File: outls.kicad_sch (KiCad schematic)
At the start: 6 parts, among them U5001 VNLD5160TR-E, U5002 VNLD5160TR-E

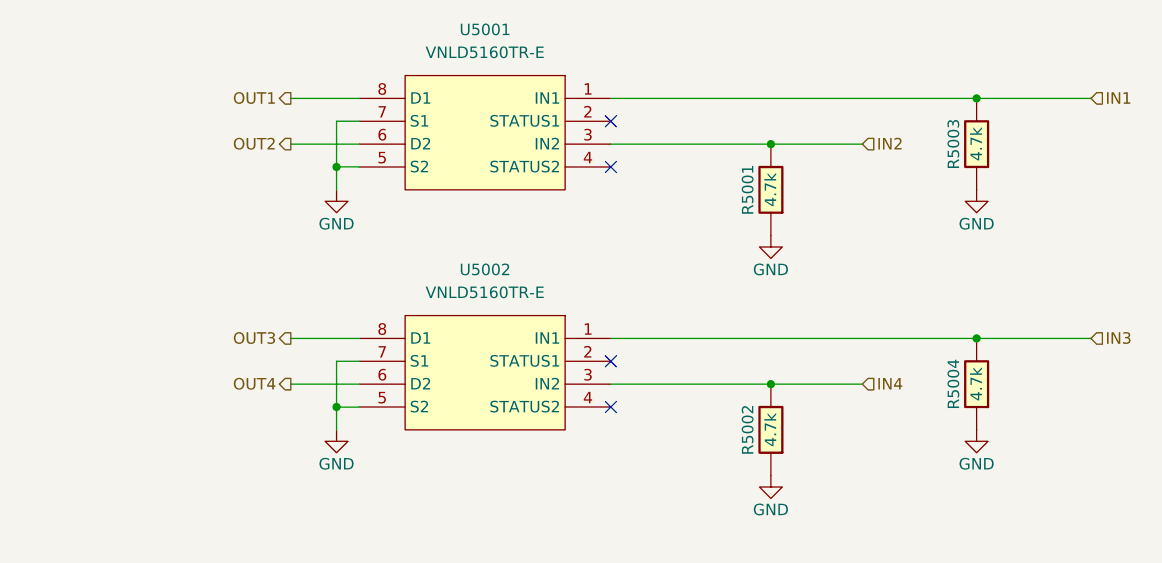
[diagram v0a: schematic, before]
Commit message: Initial schematic
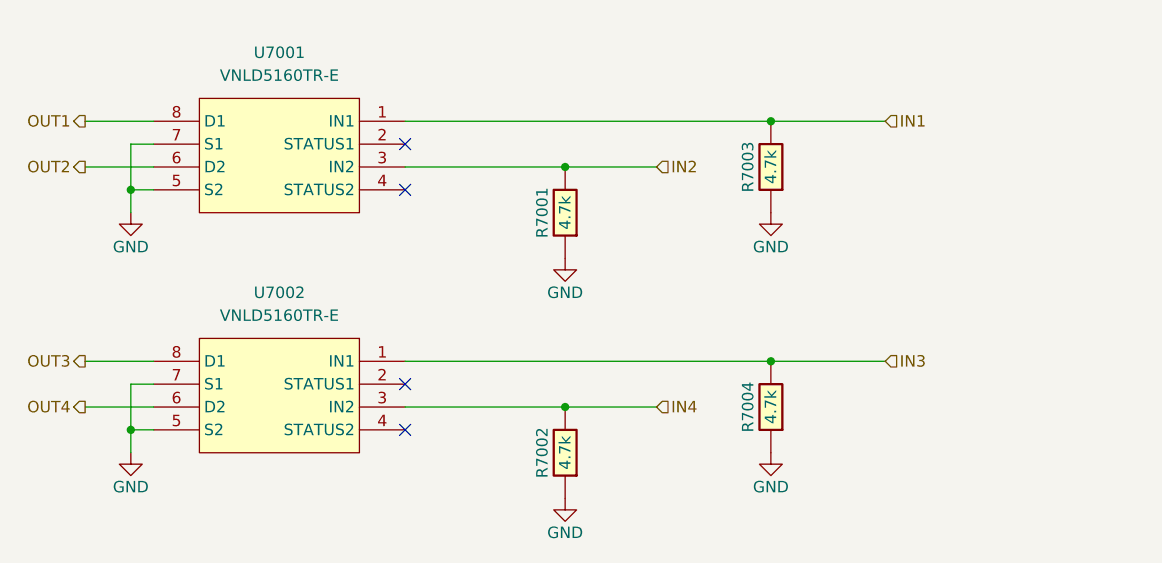
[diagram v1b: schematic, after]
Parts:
- removed R5001, R5002, R5003, R5004: 4.7k, hellen-one-common:R0603, symbol hellen-one-common:Res
- removed U5001, U5002: VNLD5160TR-E, Package_SO:SOIC-8_3.9x4.9mm_P1.27mm, symbol chips:VNLD5160
- added R7001, R7002, R7003, R7004: 4.7k, hellen-one-common:R0603, symbol hellen-one-common:Res
- added U7001, U7002: VNLD5160TR-E, Package_SO:SOIC-8_3.9x4.9mm_P1.27mm, symbol chips:VNLD5160
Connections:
- net GND: now also R7001.1, R7002.1, R7003.1, R7004.1, U7001.5 (S2), U7001.7 (S1), U7002.5 (S2), U7002.7 (S1)
- net IN1: now also R7003.2, U7001.1 (IN1)
- net IN2: now also R7001.2, U7001.3 (IN2)
- net IN3: now also R7004.2, U7002.1 (IN1)
- net IN4: now also R7002.2, U7002.3 (IN2)
- net OUT1: now also U7001.8 (D1)
- net OUT2: now also U7001.6 (D2)
- net OUT3: now also U7002.8 (D1)
- net OUT4: now also U7002.6 (D2)
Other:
- company: rusEFI.com -> (none)
- title: UAEFI -> (none)
